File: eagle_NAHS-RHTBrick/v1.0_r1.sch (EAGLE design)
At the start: 44 parts, among them IC1 ESP12S, IC2 ATTINY212-SSNR, IC3 TP4056, IC4 DW01A, IC5 HDC1080, J1 10118194-0001LF, J2 BRICK-INTERF-V3_B-SIDE, Q1 8205A, T1 PINHD_1X03_R_1, T2 PINHD_1X03_R_1, T3 PINHD_1X03_R_1

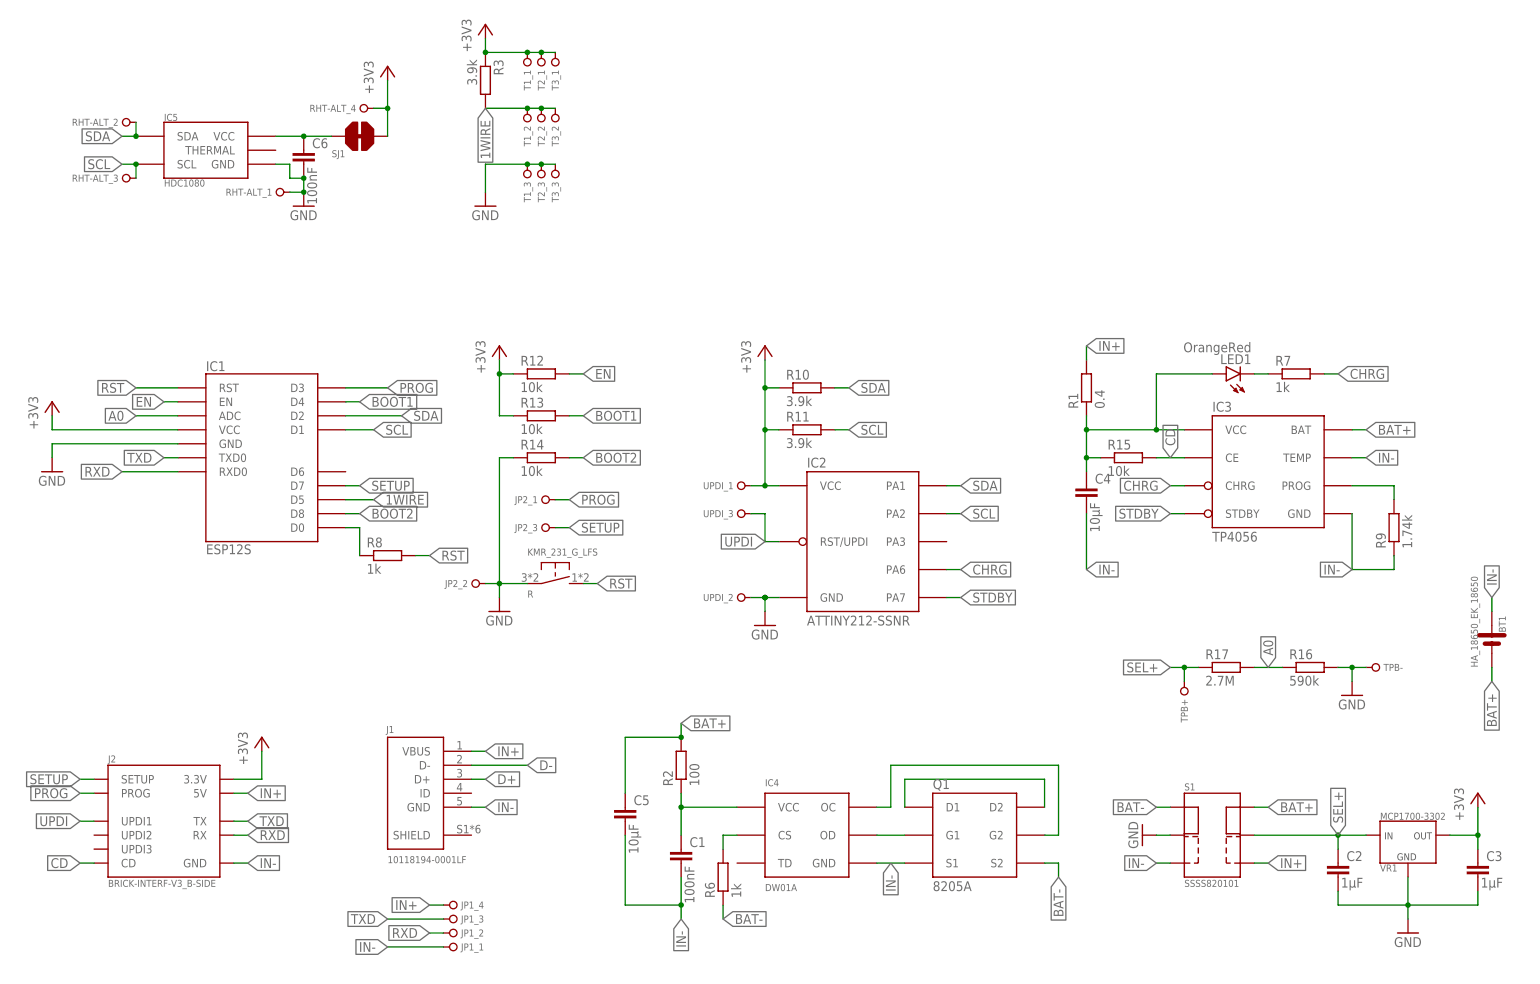
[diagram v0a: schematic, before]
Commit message: v1.0 R1 Board done
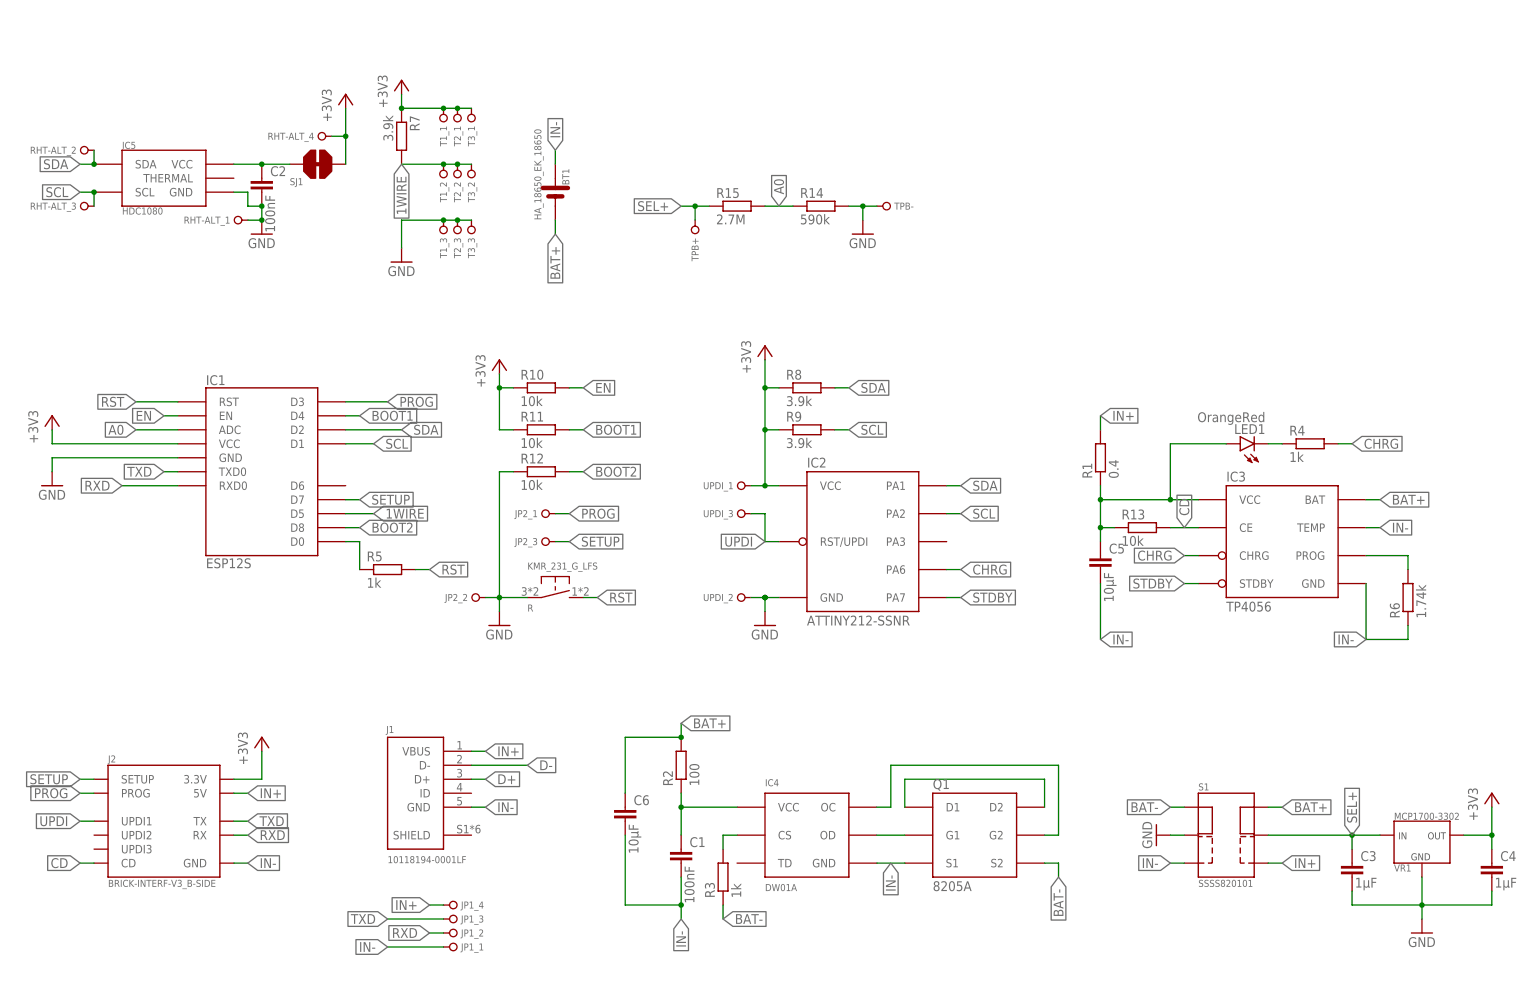
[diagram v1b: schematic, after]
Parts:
- removed R16: 590k, rcl:R-EU_R0805
- removed R17: 2.7M, rcl:R-EU_R0805
- added R4, R5: 1k, rcl:R-EU_R0805
- C2: value 1µF -> 100nF
- C4: value 10µF -> 1µF
- C6: value 100nF -> 10µF
- R10, R11: value 3.9k -> 10k
- R14: value 10k -> 590k
- R15: value 10k -> 2.7M
- R3: value 3.9k -> 1k
- R6: value 1k -> 1.74k
- R7, R8: value 1k -> 3.9k
- R9: value 1.74k -> 3.9k
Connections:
- net +3V3: now also C4.1, R7.1, R8.1, R9.1; no longer C3.1, R12.1, R13.1, R3.1
- net 1WIRE: now also R7.2; no longer R3.2
- net A0: now also R14.1, R15.2; no longer R16.1, R17.2
- net BAT+: now also C6.1; no longer C5.1
- net BAT-: now also R3.1; no longer R6.1
- net BOOT1: now also R11.2; no longer R13.2
- net BOOT2: now also R12.2; no longer R14.2
- net CD: now also R13.2; no longer R15.2
- net CHRG: now also R4.2; no longer R7.2
- net EN: now also R10.2; no longer R12.2
- net GND: now also C4.2, R12.1, R14.2; no longer C6.2, R14.1, R16.2
- net IN-: now also C6.2, R6.1; no longer C4.2, R9.1
- net N$1: now also C5.1, R13.1; no longer C4.1, R15.1
- net N$2: now also R6.2; no longer R9.2
- net N$3: now also R3.2; no longer R6.2
- net N$5: now also C2.1; no longer C6.1
- net N$7: now also R4.1; no longer R7.1
- net RST: now also R5.2; no longer R8.2
- net SCL: now also R9.2; no longer R11.2
- net SDA: now also R8.2; no longer R10.2
- net SEL+: now also C3.1, R15.1; no longer C2.1, R17.1
- net WAKE: now also R5.1; no longer R8.1
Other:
- moved on the sheet: BT1, C2, C3, C4, C5, C6, IC1, IC3, IC5, JP2_1, JP2_2, JP2_3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
